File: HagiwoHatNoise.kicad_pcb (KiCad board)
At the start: 2 copper layers, 30 x 106 mm, 37 parts, among them J1 Trig In, J2 Decay CV In, J3 Tune CV In, J4 Eurorack_Power_16pin_Shrouded, J5 Audio Out, Q1 2SC1815

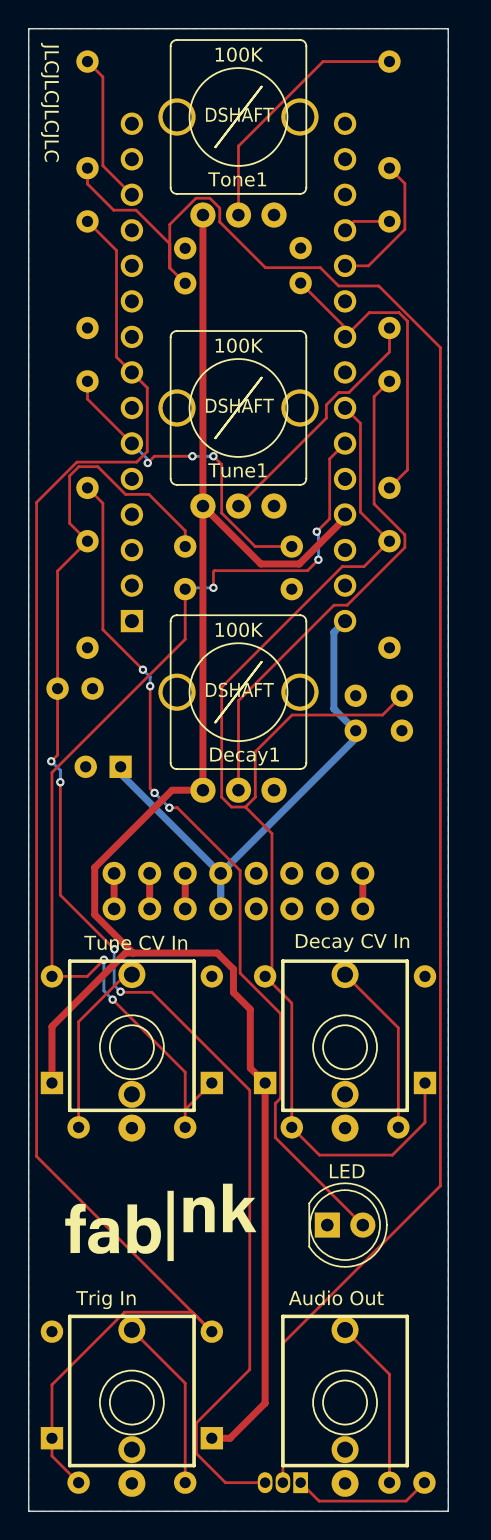
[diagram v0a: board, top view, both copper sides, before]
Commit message: v1.0 ready for production
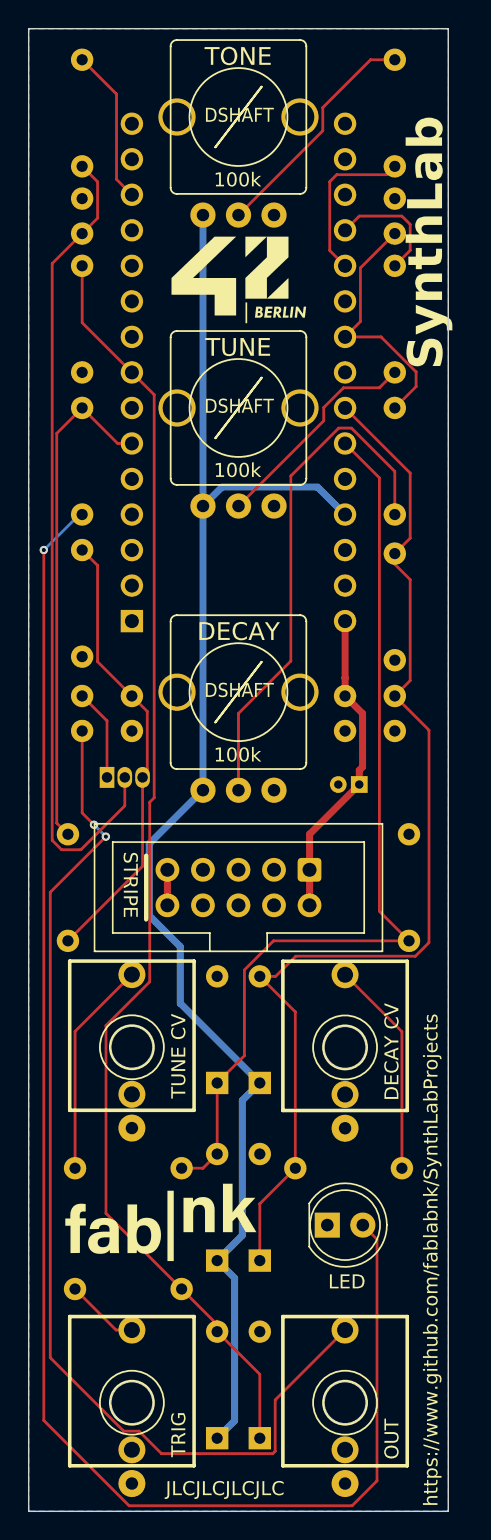
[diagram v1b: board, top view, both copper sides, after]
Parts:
- removed Decay1, Tone1, Tune1: 100K, Library:Pot_9mm_DShaft_RemovedPins4_5
- removed J1: Trig In, Library:EighthInch_PJ398SM_T_TN_S
- removed J2: Decay CV In, Library:EighthInch_PJ398SM_T_TN_S
- removed J4: Eurorack_Power_16pin_Shrouded, Library:Pins_2x08_2.54mm_TH_EuroPower_Shrouded_Minimal
- removed J5: Audio Out, Library:EighthInch_PJ398SM_T_TN_S
- added J6: TRIG, Library:EighthInch_PJ398SM_3mmNPTH, F.Cu at (58.4, 149.0)
- added J7: DECAY CV, Library:EighthInch_PJ398SM_3mmNPTH, F.Cu at (73.7, 123.6)
- added J8: TUNE CV, Library:EighthInch_PJ398SM_3mmNPTH, F.Cu at (58.4, 123.6)
- added J9: OUT, Library:EighthInch_PJ398SM_3mmNPTH, F.Cu at (73.7, 149.0)
- added RV1: 100k, Library:Pot_9mm_DShaft_RemovedPins4_5, F.Cu at (66.0, 77.9)
- added RV2: 100k, Library:Pot_9mm_DShaft_RemovedPins4_5, F.Cu at (66.0, 57.1)
- added RV3: 100k, Library:Pot_9mm_DShaft_RemovedPins4_5, F.Cu at (66.0, 98.2)
- C1: renamed from C5; value 225 -> 2.2uF
- C2: renamed from C3; value 223 -> 22nF
- C3: renamed from C4; value 332 -> 3.3nF
- C4: renamed from C1; value 101 -> 100pF
- C5: renamed from C6; value 104 -> 100nF
- C6: renamed from C7; footprint Capacitor_THT:CP_Radial_D6.3mm_P2.50mm -> Capacitor_THT:CP_Radial_D4.0mm_P1.50mm
- C7: renamed from C2; value 101 -> 100pF
- D2: renamed from D1; value B43 -> BAT43; footprint Diode_THT:D_DO-35_SOD27_P7.62mm_Horizontal -> Library:D_DO-35_SOD27_P7.62mm_Horizontal_Widened_No_K
- D3: renamed from D2; value B43 -> BAT43; footprint Diode_THT:D_DO-35_SOD27_P7.62mm_Horizontal -> Library:D_DO-35_SOD27_P7.62mm_Horizontal_Widened_No_K
- D4: renamed from D3; value B43 -> BAT43; footprint Diode_THT:D_DO-35_SOD27_P7.62mm_Horizontal -> Library:D_DO-35_SOD27_P7.62mm_Horizontal_Widened_No_K
- D5: renamed from D4; value B43 -> BAT43; footprint Diode_THT:D_DO-35_SOD27_P7.62mm_Horizontal -> Library:D_DO-35_SOD27_P7.62mm_Horizontal_Widened_No_K
- D6: renamed from D5; value B43 -> BAT43; footprint Diode_THT:D_DO-35_SOD27_P7.62mm_Horizontal -> Library:D_DO-35_SOD27_P7.62mm_Horizontal_Widened_No_K
- D7: renamed from D6; value B43 -> BAT43; footprint Diode_THT:D_DO-35_SOD27_P7.62mm_Horizontal -> Library:D_DO-35_SOD27_P7.62mm_Horizontal_Widened_No_K
- J3: value Tune CV In -> Eurorack_Power_10pin_Unshrouded; footprint Library:EighthInch_PJ398SM_T_TN_S -> Library:IDC-Header_2x05_P2.54mm_Vertical_Euro_Power_Striped_ThickerText
- R1: value 1K -> 1k
- R10: renamed from R5; value 1K -> 1k
- R11: renamed from R8; value 100K -> 100k
- R12: renamed from R6; value 1K -> 1k
- R13: renamed from R9; value 100K -> 100k
- R3: renamed from R2; value 1K -> 1k
- R4: renamed from R12; value 2.7K -> 2.7k
- R5: renamed from R13; value 100K -> 100k
- R6: renamed from R10; value 33K -> 33k
- R7: renamed from R3; value 1K -> 1k
- R8: renamed from R4; value 1K -> 1k
- R9: renamed from R7; value 100K -> 100k
- moved C1 61.3 mm to (54.9, 98.5), turned to -90 degrees
- moved Q1 52.3 mm to (56.6, 104.3), turned to 0 degrees
- moved R13 29.8 mm to (78.2, 116.0), turned to 90 degrees
- moved R4 26.1 mm to (53.8, 108.4), turned to -90 degrees
- moved J3 18.0 mm to (71.1, 110.9)
- moved D5 17.3 mm to (67.6, 138.9)
- moved D6 17.3 mm to (64.5, 138.9)
- moved C6 17.1 mm to (74.7, 104.8)
- moved R8 15.9 mm to (54.4, 140.9), turned to 0 degrees
- moved D3 14.9 mm to (67.6, 151.6)
- moved R7 9.53 mm to (77.2, 85.5), turned to 90 degrees
- moved C2 8.18 mm to (54.9, 65.4)
- moved C4 7.60 mm to (77.2, 65.4)
- moved C3 5.34 mm to (58.4, 98.5), turned to -90 degrees
- moved R9 3.20 mm to (54.9, 67.8)
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- renumbered D7 to D1, R11 to R2
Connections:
- R12 pad 1: Net-(J3-PadT) -> Net-(J8-SIG)
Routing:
- net Net-(Q1-C): track 126.1 -> 58.8 mm
- net Net-(Q1-B): track 97.6 -> 32.2 mm, vias 4 -> 0
- net Net-(J9-SIG): track 12.2 -> 76.9 mm, vias 0 -> 2
- net Net-(D1-A): track 61.5 -> 111.8 mm, vias 4 -> 1
- net +5V: track 128.4 -> 106.1 mm
- net D5: track 114.1 -> 92.7 mm
- net Net-(J8-SIG): track 0.00 -> 15.5 mm
- net A5: track 92.2 -> 78.1 mm
- net +12V: track 36.2 -> 22.4 mm
- net D3: track 23.4 -> 36.2 mm, vias 3 -> 0
- net Net-(J3-PadT): track 12.8 -> 0.00 mm
- net Net-(J6-SIG): track 12.5 -> 5.28 mm
- net A6: track 73.2 -> 67.0 mm, vias 5 -> 0
- net A0: track 3.44 -> 8.74 mm
- net A3: track 23.1 -> 18.2 mm
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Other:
- board text added: "SynthLab"
- board text added: "`NOISE & HI-HAT` ORIGINAL DESIGN BY HAGIWO"
- board text added: "https://www.github.com/fablabnk/SynthLabProjects"
- board text removed: "`NOISE & HH` ORIGINAL DESIGN BY HAGIWO"
